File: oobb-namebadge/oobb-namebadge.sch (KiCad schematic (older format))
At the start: 13 parts, among them J1 Conn_02x03_Odd_Even, J2 Conn_02x03_Odd_Even, J3 Conn_02x03_Odd_Even, J4 Conn_02x03_Odd_Even, J5 Conn_01x06, J6 Conn_02x03_Odd_Even, J7 Conn_01x01, J8 Conn_01x01, SW1 SW_SPDT, U1 AP1117-15, U2 lipo-charger-boost

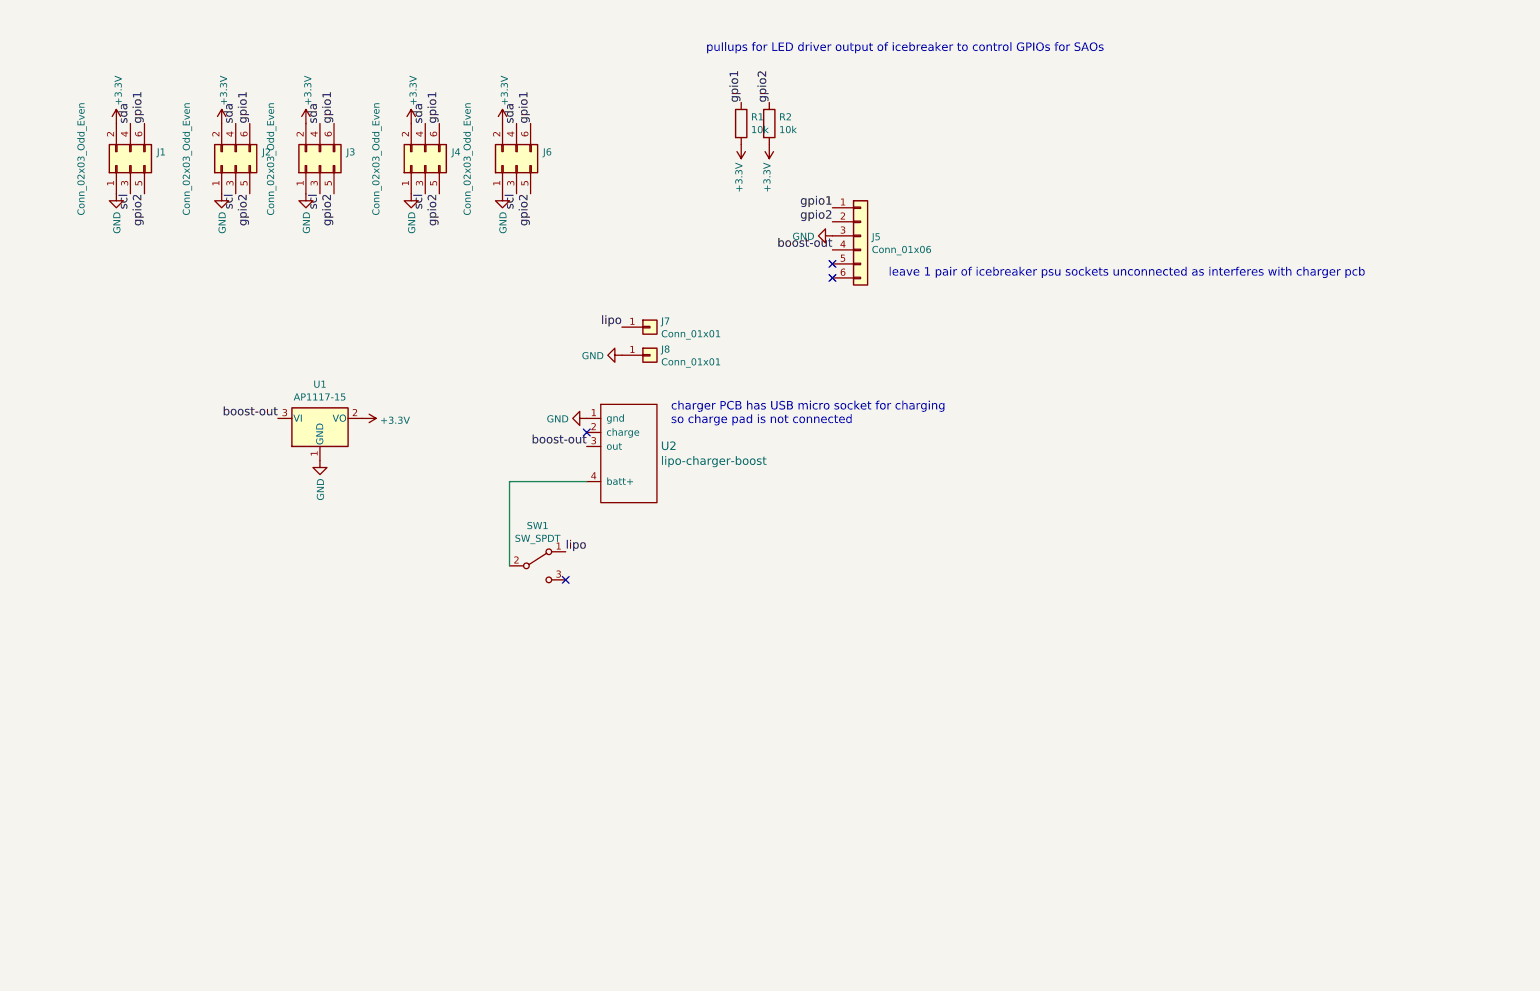
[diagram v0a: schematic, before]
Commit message: layout
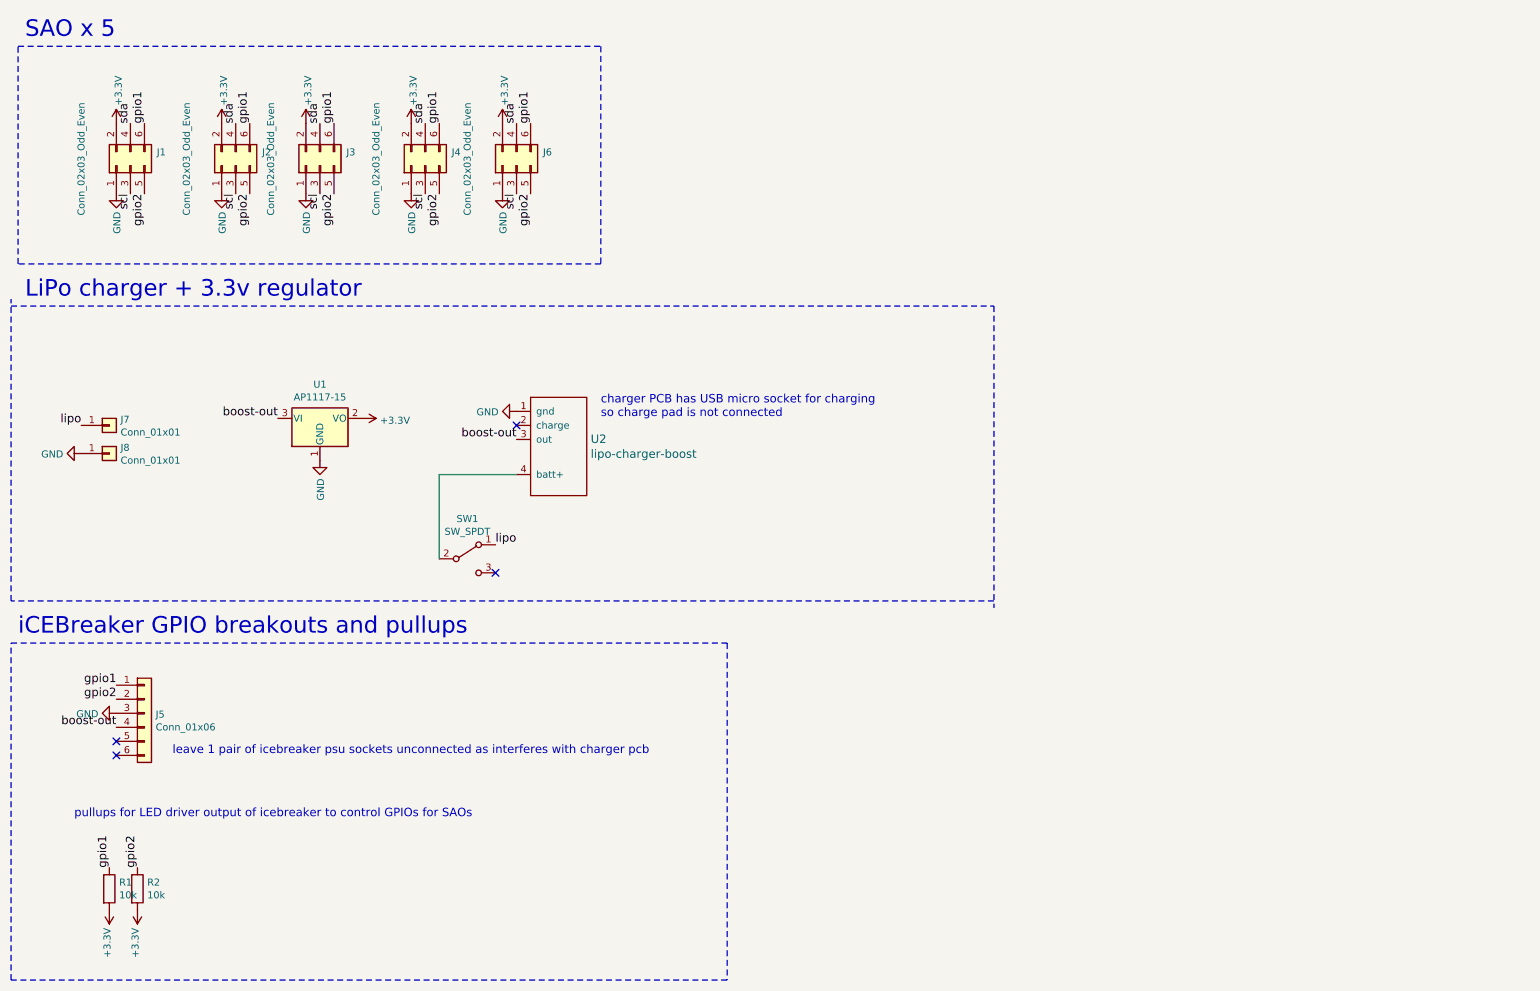
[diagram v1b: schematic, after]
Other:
- note added: "LiPo charger + 3.3v regulator\n"
- note added: "SAO x 5"
- note added: "iCEBreaker GPIO breakouts and pullups"
- moved on the sheet: J5, J7, J8, R1, R2, SW1, U2
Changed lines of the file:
@@
 L Conn_01x01 J7
 U 1 1 5D963A71
-P 5950 2900
-F 0 "J7" H 6030 2942 50  0000 L CNN
-F 1 "Conn_01x01" H 6030 2851 50  0000 L CNN
-F 2 "Measurement_Points:Measurement_Point_Square-SMD-Pad_Big" H 5950 2900 50  0001 C CNN
-F 3 "~" H 5950 2900 50  0001 C CNN
-	1    5950 2900
+P 2100 3600
+F 0 "J7" H 2180 3642 50  0000 L CNN
+F 1 "Conn_01x01" H 2180 3551 50  0000 L CNN
+F 2 "Measurement_Points:Measurement_Point_Square-SMD-Pad_Big" H 2100 3600 50  0001 C CNN
+F 3 "~" H 2100 3600 50  0001 C CNN
+	1    2100 3600
 	1    0    0    -1
 $EndComp
@@
 L Conn_01x01 J8
 U 1 1 5D963ABB
-P 5950 3100
-F 0 "J8" H 6030 3142 50  0000 L CNN
-F 1 "Conn_01x01" H 6030 3051 50  0000 L CNN
-F 2 "Measurement_Points:Measurement_Point_Square-SMD-Pad_Big" H 5950 3100 50  0001 C CNN
-F 3 "~" H 5950 3100 50  0001 C CNN
-	1    5950 3100
+P 2100 3800
+F 0 "J8" H 2180 3842 50  0000 L CNN
+F 1 "Conn_01x01" H 2180 3751 50  0000 L CNN
+F 2 "Measurement_Points:Measurement_Point_Square-SMD-Pad_Big" H 2100 3800 50  0001 C CNN
+F 3 "~" H 2100 3800 50  0001 C CNN
+	1    2100 3800
 	1    0    0    -1
 $EndComp
@@
 L lipo-charger-boost U2
 U 1 1 5D9C5C35
-P 5800 3800
-F 0 "U2" H 6028 3853 60  0000 L CNN
-F 1 "lipo-charger-boost" H 6028 3747 60  0000 L CNN
-F 2 "oobb:lipo-charger-boost" H 5800 3800 60  0001 C CNN
-F 3 "" H 5800 3800 60  0001 C CNN
-	1    5800 3800
+P 5300 3750
+F 0 "U2" H 5528 3803 60  0000 L CNN
+F 1 "lipo-charger-boost" H 5528 3697 60  0000 L CNN
+F 2 "oobb:lipo-charger-boost" H 5300 3750 60  0001 C CNN
+F 3 "" H 5300 3750 60  0001 C CNN
+	1    5300 3750
 	1    0    0    -1
 $EndComp
@@
 L GND #PWR011
 U 1 1 5D9C5C9F
-P 5500 3550
-F 0 "#PWR011" H 5500 3300 50  0001 C CNN
-F 1 "GND" V 5505 3422 50  0000 R CNN
-F 2 "" H 5500 3550 50  0001 C CNN
-F 3 "" H 5500 3550 50  0001 C CNN
-	1    5500 3550
+P 5000 3500
+F 0 "#PWR011" H 5000 3250 50  0001 C CNN
+F 1 "GND" V 5005 3372 50  0000 R CNN
+F 2 "" H 5000 3500 50  0001 C CNN
+F 3 "" H 5000 3500 50  0001 C CNN
+	1    5000 3500
 	0    1    1    0
 $EndComp
-NoConn ~ 5500 3650
+NoConn ~ 5000 3600
 $Comp
 L AP1117-15 U1
@@
 L SW_SPDT SW1
 U 1 1 5D9C5F59
-P 5150 4600
-F 0 "SW1" H 5150 4885 50  0000 C CNN
-F 1 "SW_SPDT" H 5150 4794 50  0000 C CNN
-F 2 "Buttons_Switches_SMD:SW_SPDT_CK-JS102011SAQN" H 5150 4600 50  0001 C CNN
-F 3 "" H 5150 4600 50  0001 C CNN
-F 4 "2320017 " H 5150 4600 60  0001 C CNN "farnell #"
-F 5 "Value" H 5150 4600 60  0001 C CNN "supplier"
-F 6 "Value" H 5150 4600 60  0001 C CNN "supplier PN"
-F 7 "Value" H 5150 4600 60  0001 C CNN "MOQ"
-F 8 "Value" H 5150 4600 60  0001 C CNN "leadtime"
-	1    5150 4600
+P 4650 4550
+F 0 "SW1" H 4650 4835 50  0000 C CNN
+F 1 "SW_SPDT" H 4650 4744 50  0000 C CNN
+F 2 "Buttons_Switches_SMD:SW_SPDT_CK-JS102011SAQN" H 4650 4550 50  0001 C CNN
+F 3 "" H 4650 4550 50  0001 C CNN
+F 4 "2320017 " H 4650 4550 60  0001 C CNN "farnell #"
+F 5 "Value" H 4650 4550 60  0001 C CNN "supplier"
+F 6 "Value" H 4650 4550 60  0001 C CNN "supplier PN"
+F 7 "Value" H 4650 4550 60  0001 C CNN "MOQ"
+F 8 "Value" H 4650 4550 60  0001 C CNN "leadtime"
+	1    4650 4550
 	1    0    0    -1
 $EndComp
@@
 L GND #PWR012
 U 1 1 5D9C6130
-P 5750 3100
-F 0 "#PWR012" H 5750 2850 50  0001 C CNN
-F 1 "GND" V 5755 2972 50  0000 R CNN
-F 2 "" H 5750 3100 50  0001 C CNN
-F 3 "" H 5750 3100 50  0001 C CNN
-	1    5750 3100
+P 1900 3800
+F 0 "#PWR012" H 1900 3550 50  0001 C CNN
+F 1 "GND" V 1905 3672 50  0000 R CNN
+F 2 "" H 1900 3800 50  0001 C CNN
+F 3 "" H 1900 3800 50  0001 C CNN
+	1    1900 3800
 	0    1    1    0
 $EndComp
-Text Label 5750 2900 2    60   ~ 0
+Text Label 1900 3600 2    60   ~ 0
 lipo
-Text Label 5350 4500 0    60   ~ 0
+Text Label 4850 4450 0    60   ~ 0
 lipo
 $Comp
@@
 	1    0    0    -1
 $EndComp
-Text Label 5500 3750 2    60   ~ 0
+Text Label 5000 3700 2    60   ~ 0
 boost-out
 Text Label 3300 3550 2    60   ~ 0
 boost-out
 Wire Wire Line
-	4950 4600 4950 4000
+	4450 4550 4450 3950
 Wire Wire Line
-	4950 4000 5500 4000
-NoConn ~ 5350 4700
+	4450 3950 5000 3950
+NoConn ~ 4850 4650
 Text Label 2250 1450 1    60   ~ 0
 sda
@@
 Text Label 5100 1950 3    60   ~ 0
 gpio2
-Text Label 7250 2050 2    60   ~ 0
-gpio1
-Text Label 7250 2150 2    60   ~ 0
-gpio2
-Text Label 7250 2350 2    60   ~ 0
+Text Label 2150 5450 2    60   ~ 0
+gpio1
+Text Label 2150 5550 2    60   ~ 0
+gpio2
+Text Label 2150 5750 2    60   ~ 0
 boost-out
 $Comp
 L GND #PWR013
 U 1 1 5D9C7066
-P 7250 2250
-F 0 "#PWR013" H 7250 2000 50  0001 C CNN
-F 1 "GND" V 7255 2122 50  0000 R CNN
-F 2 "" H 7250 2250 50  0001 C CNN
-F 3 "" H 7250 2250 50  0001 C CNN
-	1    7250 2250
+P 2150 5650
+F 0 "#PWR013" H 2150 5400 50  0001 C CNN
+F 1 "GND" V 2155 5522 50  0000 R CNN
+F 2 "" H 2150 5650 50  0001 C CNN
+F 3 "" H 2150 5650 50  0001 C CNN
+	1    2150 5650
 	0    1    1    0
 $EndComp
@@
 L Conn_01x06 J5
 U 1 1 5D9C72D7
-P 7450 2250
-F 0 "J5" H 7530 2242 50  0000 L CNN
-F 1 "Conn_01x06" H 7530 2151 50  0000 L CNN
-F 2 "oobb:icebreaker" H 7450 2250 50  0001 C CNN
-F 3 "~" H 7450 2250 50  0001 C CNN
-	1    7450 2250
-	1    0    0    -1
-$EndComp
-NoConn ~ 7250 2450
-NoConn ~ 7250 2550
-Text Notes 6100 3600 0    60   ~ 0
+P 2350 5650
+F 0 "J5" H 2430 5642 50  0000 L CNN
+F 1 "Conn_01x06" H 2430 5551 50  0000 L CNN
+F 2 "oobb:icebreaker" H 2350 5650 50  0001 C CNN
+F 3 "~" H 2350 5650 50  0001 C CNN
+	1    2350 5650
+	1    0    0    -1
+$EndComp
+NoConn ~ 2150 5850
+NoConn ~ 2150 5950
+Text Notes 5600 3550 0    60   ~ 0
 charger PCB has USB micro socket for charging\nso charge pad is not connected
-Text Notes 6100 5200 0    60   ~ 0
+Text Notes 5600 5200 0    60   ~ 0
 \n
-Text Notes 7650 2550 0    60   ~ 0
+Text Notes 2550 5950 0    60   ~ 0
 leave 1 pair of icebreaker psu sockets unconnected as interferes with charger pcb
 $Comp
 L R R1
 U 1 1 5D9F3122
-P 6600 1450
-F 0 "R1" H 6670 1496 50  0000 L CNN
-F 1 "10k" H 6670 1405 50  0000 L CNN
-F 2 "Resistors_SMD:R_0805_HandSoldering" V 6530 1450 50  0001 C CNN
-F 3 "" H 6600 1450 50  0001 C CNN
-F 4 "Value" H 6600 1450 60  0001 C CNN "supplier"
-F 5 "Value" H 6600 1450 60  0001 C CNN "supplier PN"
-F 6 "Value" H 6600 1450 60  0001 C CNN "MOQ"
-F 7 "Value" H 6600 1450 60  0001 C CNN "leadtime"
-	1    6600 1450
+P 2100 6900
+F 0 "R1" H 2170 6946 50  0000 L CNN
+F 1 "10k" H 2170 6855 50  0000 L CNN
+F 2 "Resistors_SMD:R_0805_HandSoldering" V 2030 6900 50  0001 C CNN
+F 3 "" H 2100 6900 50  0001 C CNN
+F 4 "Value" H 2100 6900 60  0001 C CNN "supplier"
+F 5 "Value" H 2100 6900 60  0001 C CNN "supplier PN"
+F 6 "Value" H 2100 6900 60  0001 C CNN "MOQ"
+F 7 "Value" H 2100 6900 60  0001 C CNN "leadtime"
+	1    2100 6900
 	1    0    0    -1
 $EndComp
@@
 L R R2
 U 1 1 5D9F317E
-P 6800 1450
-F 0 "R2" H 6870 1496 50  0000 L CNN
-F 1 "10k" H 6870 1405 50  0000 L CNN
-F 2 "Resistors_SMD:R_0805_HandSoldering" V 6730 1450 50  0001 C CNN
-F 3 "" H 6800 1450 50  0001 C CNN
-F 4 "Value" H 6800 1450 60  0001 C CNN "supplier"
-F 5 "Value" H 6800 1450 60  0001 C CNN "supplier PN"
-F 6 "Value" H 6800 1450 60  0001 C CNN "MOQ"
-F 7 "Value" H 6800 1450 60  0001 C CNN "leadtime"
-	1    6800 1450
-	1    0    0    -1
-$EndComp
-Text Label 6600 1300 1    60   ~ 0
-gpio1
-Text Label 6800 1300 1    60   ~ 0
+P 2300 6900
+F 0 "R2" H 2370 6946 50  0000 L CNN
+F 1 "10k" H 2370 6855 50  0000 L CNN
+F 2 "Resistors_SMD:R_0805_HandSoldering" V 2230 6900 50  0001 C CNN
+F 3 "" H 2300 6900 50  0001 C CNN
+F 4 "Value" H 2300 6900 60  0001 C CNN "supplier"
+F 5 "Value" H 2300 6900 60  0001 C CNN "supplier PN"
+F 6 "Value" H 2300 6900 60  0001 C CNN "MOQ"
+F 7 "Value" H 2300 6900 60  0001 C CNN "leadtime"
+	1    2300 6900
+	1    0    0    -1
+$EndComp
+Text Label 2100 6750 1    60   ~ 0
+gpio1
+Text Label 2300 6750 1    60   ~ 0
 gpio2
 $Comp
 L +3.3V #PWR014
 U 1 1 5D9F3332
-P 6600 1600
-F 0 "#PWR014" H 6600 1450 50  0001 C CNN
-F 1 "+3.3V" V 6615 1728 50  0000 L CNN
-F 2 "" H 6600 1600 50  0001 C CNN
-F 3 "" H 6600 1600 50  0001 C CNN
-	1    6600 1600
+P 2100 7050
+F 0 "#PWR014" H 2100 6900 50  0001 C CNN
+F 1 "+3.3V" V 2115 7178 50  0000 L CNN
+F 2 "" H 2100 7050 50  0001 C CNN
+F 3 "" H 2100 7050 50  0001 C CNN
+	1    2100 7050
 	-1   0    0    1
 $EndComp
@@
 L +3.3V #PWR017
 U 1 1 5D9F3398
-P 6800 1600
-F 0 "#PWR017" H 6800 1450 50  0001 C CNN
-F 1 "+3.3V" V 6815 1728 50  0000 L CNN
-F 2 "" H 6800 1600 50  0001 C CNN
-F 3 "" H 6800 1600 50  0001 C CNN
-	1    6800 1600
+P 2300 7050
+F 0 "#PWR017" H 2300 6900 50  0001 C CNN
+F 1 "+3.3V" V 2315 7178 50  0000 L CNN
+F 2 "" H 2300 7050 50  0001 C CNN
+F 3 "" H 2300 7050 50  0001 C CNN
+	1    2300 7050
 	-1   0    0    1
 $EndComp
-Text Notes 6350 950  0    60   ~ 0
+Text Notes 1850 6400 0    60   ~ 0
 pullups for LED driver output of icebreaker to control GPIOs for SAOs\n
+Wire Notes Line
+	1450 900  5600 900
+Wire Notes Line
+	5600 900  5600 2450
+Wire Notes Line
+	5600 2450 1450 2450
+Wire Notes Line
+	1450 2450 1450 900
+Wire Notes Line
+	1400 2750 8400 2750
+Wire Notes Line
+	8400 2750 8400 4900
+Wire Notes Line
+	8400 4850 1400 4850
+Wire Notes Line
+	1400 4850 1400 2700
+Wire Notes Line
+	1400 5150 6500 5150
+Wire Notes Line
+	6500 5150 6500 7550
+Wire Notes Line
+	6500 7550 1400 7550
+Wire Notes Line
+	1400 7550 1400 5150
+Text Notes 1500 850  0    118  ~ 0
+SAO x 5
+Text Notes 1500 2700 0    118  ~ 0
+LiPo charger + 3.3v regulator\n
+Text Notes 1450 5100 0    118  ~ 0
+iCEBreaker GPIO breakouts and pullups
 $EndSCHEMATC
